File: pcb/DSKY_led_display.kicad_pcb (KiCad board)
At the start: 4 copper layers, 63.5 x 107.9 mm, 239 parts, among them J1 105133-0001, J2 3221-10-0300-00-TR, J3 TSM-104-01-L-SV, SW1 KMR241NG, U1 AP2204K-3.3, U2 LP5036, U3 LP5036, U4 LP5036, U5 LP5036, U6 ATSAMD21E18A-A, U7 LP5036, U8 LP5036, U9 TCA9543ADR

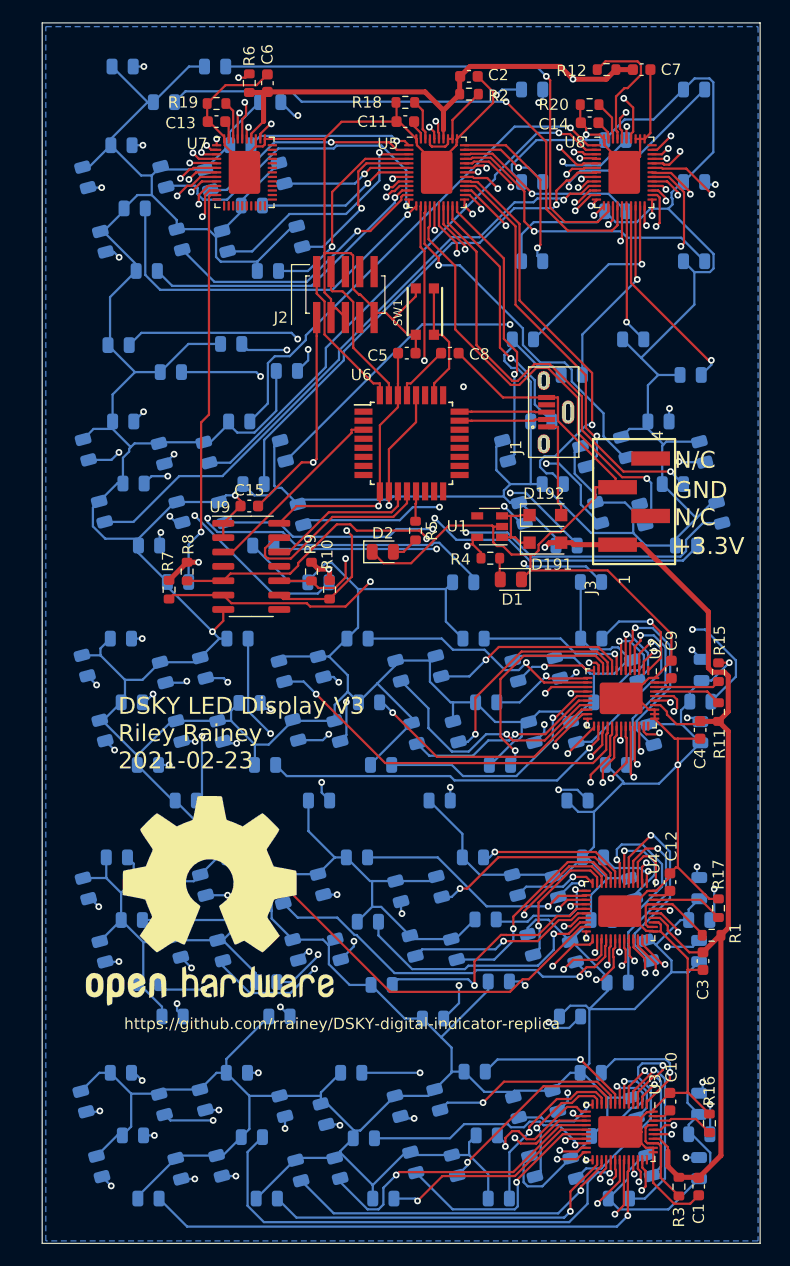
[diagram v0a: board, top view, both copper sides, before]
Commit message: V4 board
Version 4 of the PCB
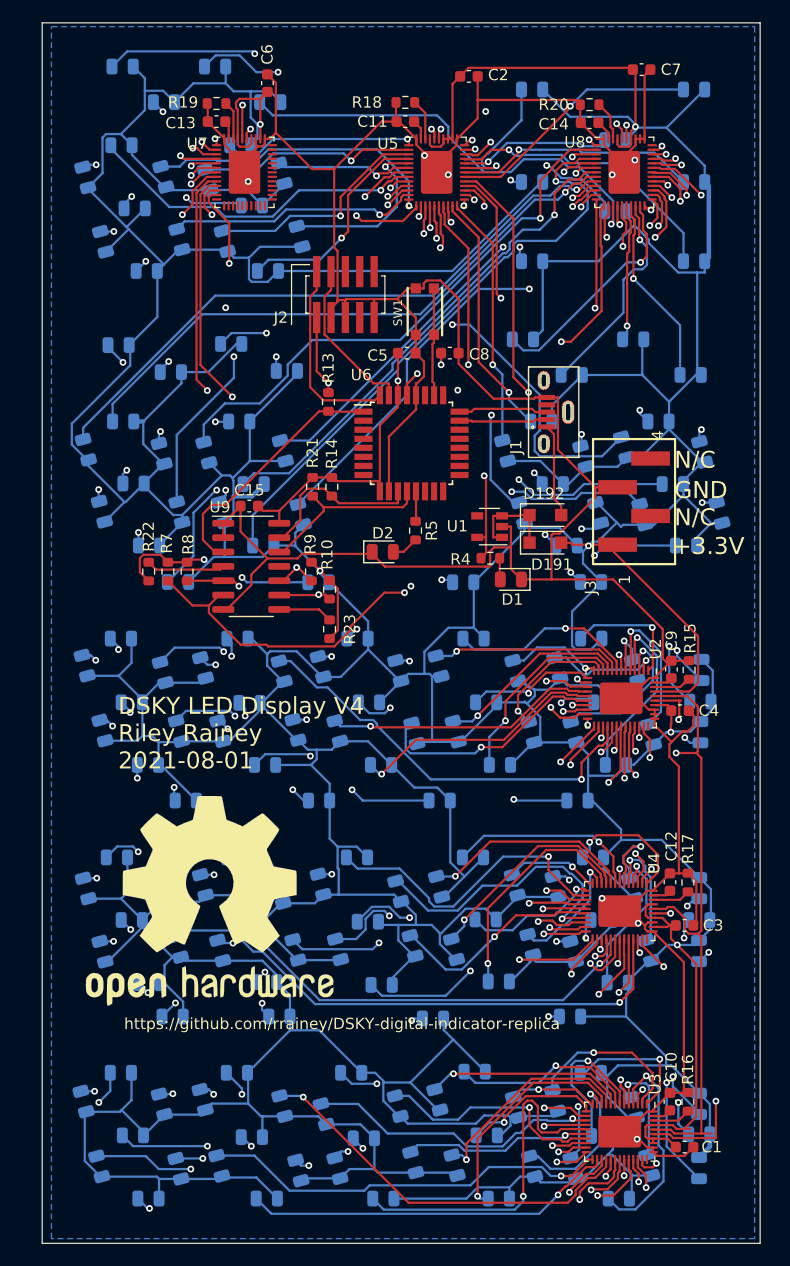
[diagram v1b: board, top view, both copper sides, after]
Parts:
- removed R1, R11, R12, R2, R3, R6: 4.7K, Resistor_SMD:R_0603_1608Metric
- added R13: 0K, Resistor_SMD:R_0603_1608Metric, F.Cu at (59.2, 66.5)
- added R14: 1K, Resistor_SMD:R_0603_1608Metric, F.Cu at (59.5, 74.0)
- added R21: 1K, Resistor_SMD:R_0603_1608Metric, F.Cu at (57.8, 74.0)
- added R22: 1K, Resistor_SMD:R_0603_1608Metric, F.Cu at (43.3, 81.5)
- added R23: 1K, Resistor_SMD:R_0603_1608Metric, F.Cu at (59.3, 86.6)
- moved C1 3.71 mm to (90.7, 132.4), turned to 0 degrees
- moved C3 3.55 mm to (90.7, 112.8), turned to 0 degrees
- moved R17 3.53 mm to (91.0, 109.0)
- moved R16 2.69 mm to (91.0, 128.4)
- moved R15 2.61 mm to (91.1, 90.2)
- moved C4 2.46 mm to (90.3, 93.8), turned to 0 degrees
- moved R7 1.60 mm to (45.0, 81.5)
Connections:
- D10 pad 1: GND -> g0bus1
- D10 pad 2: g0bus1 -> VCC
- D100 pad 1: GND -> abus32
- D100 pad 2: abus32 -> VCC
- D101 pad 1: GND -> abus3
- D101 pad 2: abus3 -> VCC
- D102 pad 1: GND -> sabus2
- D102 pad 2: sabus2 -> VCC
- D103 pad 1: GND -> abus10
- D103 pad 2: abus10 -> VCC
- D104 pad 1: GND -> abus17
- D104 pad 2: abus17 -> VCC
- D105 pad 1: GND -> abus24
- D105 pad 2: abus24 -> VCC
- D106 pad 1: GND -> abus31
- D106 pad 2: abus31 -> VCC
- D107 pad 1: GND -> g5bus0
- D107 pad 2: g5bus0 -> VCC
- D108 pad 1: GND -> g5bus1
- D108 pad 2: g5bus1 -> VCC
- D109 pad 1: GND -> g5bus2
- D109 pad 2: g5bus2 -> VCC
- D11 pad 1: GND -> g0bus6
- D11 pad 2: g0bus6 -> VCC
- D110 pad 1: GND -> g5bus3
- D110 pad 2: g5bus3 -> VCC
- D111 pad 1: GND -> bbus0
- D111 pad 2: bbus0 -> VCC
- D112 pad 1: GND -> sbbus0
- D112 pad 2: sbbus0 -> VCC
- D113 pad 1: GND -> bbus7
- D113 pad 2: bbus7 -> VCC
- D114 pad 1: GND -> bbus14
- D114 pad 2: bbus14 -> VCC
- D115 pad 1: GND -> bbus21
- D115 pad 2: bbus21 -> VCC
- D116 pad 1: GND -> bbus28
- D116 pad 2: bbus28 -> VCC
- D117 pad 1: GND -> bbus5
- D117 pad 2: bbus5 -> VCC
- D118 pad 1: GND -> bbus1
- D118 pad 2: bbus1 -> VCC
- D119 pad 1: GND -> bbus12
- D119 pad 2: bbus12 -> VCC
- D12 pad 1: GND -> g0bus5
- D12 pad 2: g0bus5 -> VCC
- D120 pad 1: GND -> bbus19
- D120 pad 2: bbus19 -> VCC
- D121 pad 1: GND -> bbus8
- D121 pad 2: bbus8 -> VCC
- D122 pad 1: GND -> bbus15
- D122 pad 2: bbus15 -> VCC
- D123 pad 1: GND -> bbus26
- D123 pad 2: bbus26 -> VCC
- D124 pad 1: GND -> bbus33
- D124 pad 2: bbus33 -> VCC
- D125 pad 1: GND -> bbus22
- D125 pad 2: bbus22 -> VCC
- D126 pad 1: GND -> bbus29
- D126 pad 2: bbus29 -> VCC
- D127 pad 1: GND -> sbbus1
- D127 pad 2: sbbus1 -> VCC
- D128 pad 1: GND -> bbus6
- D128 pad 2: bbus6 -> VCC
- D129 pad 1: GND -> bbus13
- D129 pad 2: bbus13 -> VCC
- D13 pad 1: GND -> g0bus4
- D13 pad 2: g0bus4 -> VCC
- D130 pad 1: GND -> bbus20
- D130 pad 2: bbus20 -> VCC
- D131 pad 1: GND -> bbus27
- D131 pad 2: bbus27 -> VCC
- D132 pad 1: GND -> bbus34
- D132 pad 2: bbus34 -> VCC
- D133 pad 1: GND -> bbus2
- D133 pad 2: bbus2 -> VCC
- D134 pad 1: GND -> bbus4
- D134 pad 2: bbus4 -> VCC
- D135 pad 1: GND -> bbus9
- D135 pad 2: bbus9 -> VCC
- D136 pad 1: GND -> bbus16
- D136 pad 2: bbus16 -> VCC
- D137 pad 1: GND -> bbus11
- D137 pad 2: bbus11 -> VCC
- D138 pad 1: GND -> bbus18
- D138 pad 2: bbus18 -> VCC
- D139 pad 1: GND -> bbus23
- D139 pad 2: bbus23 -> VCC
- D14 pad 1: GND -> g0bus7
- D14 pad 2: g0bus7 -> VCC
- D140 pad 1: GND -> bbus30
- D140 pad 2: bbus30 -> VCC
- D141 pad 1: GND -> bbus25
- D141 pad 2: bbus25 -> VCC
- D142 pad 1: GND -> bbus32
- D142 pad 2: bbus32 -> VCC
- D143 pad 1: GND -> sbbus2
- D143 pad 2: sbbus2 -> VCC
- D144 pad 1: GND -> bbus3
- D144 pad 2: bbus3 -> VCC
- D145 pad 1: GND -> bbus10
- D145 pad 2: bbus10 -> VCC
- D146 pad 1: GND -> bbus17
- D146 pad 2: bbus17 -> VCC
- D147 pad 1: GND -> bbus24
- D147 pad 2: bbus24 -> VCC
- D148 pad 1: GND -> bbus31
- D148 pad 2: bbus31 -> VCC
- D149 pad 1: GND -> g6bus0
- D149 pad 2: g6bus0 -> VCC
- D15 pad 1: GND -> dbus0
- D15 pad 2: dbus0 -> VCC
- D150 pad 1: GND -> g6bus1
- D150 pad 2: g6bus1 -> VCC
- D151 pad 1: GND -> g6bus2
- D151 pad 2: g6bus2 -> VCC
- D152 pad 1: GND -> g6bus3
- D152 pad 2: g6bus3 -> VCC
- D153 pad 1: GND -> scbus0
- D153 pad 2: scbus0 -> VCC
- D154 pad 1: GND -> cbus0
- D154 pad 2: cbus0 -> VCC
- D155 pad 1: GND -> cbus7
- D155 pad 2: cbus7 -> VCC
- D156 pad 1: GND -> cbus14
- D156 pad 2: cbus14 -> VCC
- D157 pad 1: GND -> cbus21
- D157 pad 2: cbus21 -> VCC
- D158 pad 1: GND -> cbus28
- D158 pad 2: cbus28 -> VCC
- D159 pad 1: GND -> cbus5
- D159 pad 2: cbus5 -> VCC
- D16 pad 1: GND -> dbus7
- D16 pad 2: dbus7 -> VCC
- D160 pad 1: GND -> cbus1
- D160 pad 2: cbus1 -> VCC
- D161 pad 1: GND -> cbus12
- D161 pad 2: cbus12 -> VCC
- D162 pad 1: GND -> cbus19
- D162 pad 2: cbus19 -> VCC
- D163 pad 1: GND -> scbus1
- D163 pad 2: scbus1 -> VCC
- D164 pad 1: GND -> cbus8
- D164 pad 2: cbus8 -> VCC
- D165 pad 1: GND -> cbus15
- D165 pad 2: cbus15 -> VCC
- D166 pad 1: GND -> cbus26
- D166 pad 2: cbus26 -> VCC
- D167 pad 1: GND -> cbus33
- D167 pad 2: cbus33 -> VCC
- D168 pad 1: GND -> cbus22
- D168 pad 2: cbus22 -> VCC
- D169 pad 1: GND -> cbus29
- D169 pad 2: cbus29 -> VCC
- D17 pad 1: GND -> dbus5
- D17 pad 2: dbus5 -> VCC
- D170 pad 1: GND -> cbus6
- D170 pad 2: cbus6 -> VCC
- D171 pad 1: GND -> cbus13
- D171 pad 2: cbus13 -> VCC
- D172 pad 1: GND -> cbus20
- D172 pad 2: cbus20 -> VCC
- D173 pad 1: GND -> cbus27
- D173 pad 2: cbus27 -> VCC
- D174 pad 1: GND -> cbus34
- D174 pad 2: cbus34 -> VCC
- D175 pad 1: GND -> cbus2
- D175 pad 2: cbus2 -> VCC
- D176 pad 1: GND -> scbus2
- D176 pad 2: scbus2 -> VCC
- D177 pad 1: GND -> cbus4
- D177 pad 2: cbus4 -> VCC
- D178 pad 1: GND -> cbus9
- D178 pad 2: cbus9 -> VCC
- D179 pad 1: GND -> cbus16
- D179 pad 2: cbus16 -> VCC
- D18 pad 1: GND -> dbus12
- D18 pad 2: dbus12 -> VCC
- D180 pad 1: GND -> cbus11
- D180 pad 2: cbus11 -> VCC
- D181 pad 1: GND -> cbus18
- D181 pad 2: cbus18 -> VCC
- D182 pad 1: GND -> cbus23
- D182 pad 2: cbus23 -> VCC
- D183 pad 1: GND -> cbus30
- D183 pad 2: cbus30 -> VCC
- D184 pad 1: GND -> cbus25
- D184 pad 2: cbus25 -> VCC
- D185 pad 1: GND -> cbus32
- D185 pad 2: cbus32 -> VCC
- D186 pad 1: GND -> cbus3
- D186 pad 2: cbus3 -> VCC
- D187 pad 1: GND -> cbus10
- D187 pad 2: cbus10 -> VCC
- D188 pad 1: GND -> cbus17
- D188 pad 2: cbus17 -> VCC
- D189 pad 1: GND -> cbus24
- D189 pad 2: cbus24 -> VCC
- D19 pad 1: GND -> dbus1
- D19 pad 2: dbus1 -> VCC
- D190 pad 1: GND -> cbus31
- D190 pad 2: cbus31 -> VCC
- D20 pad 1: GND -> dbus8
- D20 pad 2: dbus8 -> VCC
- D21 pad 1: GND -> dbus6
- D21 pad 2: dbus6 -> VCC
- D22 pad 1: GND -> dbus13
- D22 pad 2: dbus13 -> VCC
- D23 pad 1: GND -> dbus2
- D23 pad 2: dbus2 -> VCC
- D24 pad 1: GND -> dbus9
- D24 pad 2: dbus9 -> VCC
- D25 pad 1: GND -> dbus4
- D25 pad 2: dbus4 -> VCC
- D26 pad 1: GND -> dbus11
- D26 pad 2: dbus11 -> VCC
- D27 pad 1: GND -> dbus3
- D27 pad 2: dbus3 -> VCC
- D28 pad 1: GND -> dbus10
- D28 pad 2: dbus10 -> VCC
- D29 pad 1: GND -> g2bus0
- D29 pad 2: g2bus0 -> VCC
- D3 pad 1: GND -> g0bus0
- D3 pad 2: g0bus0 -> VCC
- D30 pad 1: GND -> g2bus3
- D30 pad 2: g2bus3 -> VCC
- D31 pad 1: GND -> g3bus0
- D31 pad 2: g3bus0 -> VCC
- D32 pad 1: GND -> g3bus3
- D32 pad 2: g3bus3 -> VCC
- D33 pad 1: GND -> g2bus1
- D33 pad 2: g2bus1 -> VCC
- D34 pad 1: GND -> g2bus2
- D34 pad 2: g2bus2 -> VCC
- D35 pad 1: GND -> g3bus1
- D35 pad 2: g3bus1 -> VCC
- D36 pad 1: GND -> g3bus2
- D36 pad 2: g3bus2 -> VCC
- D37 pad 1: GND -> ebus0
- D37 pad 2: ebus0 -> VCC
- D38 pad 1: GND -> ebus7
- D38 pad 2: ebus7 -> VCC
- D39 pad 1: GND -> fbus0
- D39 pad 2: fbus0 -> VCC
- D4 pad 1: GND -> g0bus2
- D4 pad 2: g0bus2 -> VCC
- D40 pad 1: GND -> fbus7
- D40 pad 2: fbus7 -> VCC
- D41 pad 1: GND -> ebus5
- D41 pad 2: ebus5 -> VCC
- D42 pad 1: GND -> ebus12
- D42 pad 2: ebus12 -> VCC
- D43 pad 1: GND -> ebus1
- D43 pad 2: ebus1 -> VCC
- D44 pad 1: GND -> ebus8
- D44 pad 2: ebus8 -> VCC
- D45 pad 1: GND -> fbus5
- D45 pad 2: fbus5 -> VCC
- D46 pad 1: GND -> fbus12
- D46 pad 2: fbus12 -> VCC
- D47 pad 1: GND -> fbus1
- D47 pad 2: fbus1 -> VCC
- D48 pad 1: GND -> fbus8
- D48 pad 2: fbus8 -> VCC
- D49 pad 1: GND -> ebus6
- D49 pad 2: ebus6 -> VCC
- D5 pad 1: GND -> g1bus0
- D5 pad 2: g1bus0 -> VCC
- D50 pad 1: GND -> ebus13
- D50 pad 2: ebus13 -> VCC
- D51 pad 1: GND -> fbus6
- D51 pad 2: fbus6 -> VCC
- D52 pad 1: GND -> fbus13
- D52 pad 2: fbus13 -> VCC
- D53 pad 1: GND -> ebus2
- D53 pad 2: ebus2 -> VCC
- D54 pad 1: GND -> ebus9
- D54 pad 2: ebus9 -> VCC
- D55 pad 1: GND -> ebus4
- D55 pad 2: ebus4 -> VCC
- D56 pad 1: GND -> VCC
- D57 pad 1: GND -> fbus2
- D57 pad 2: fbus2 -> VCC
- D58 pad 1: GND -> fbus9
- D58 pad 2: fbus9 -> VCC
- D59 pad 1: GND -> fbus4
- D59 pad 2: fbus4 -> VCC
- D6 pad 1: GND -> g1bus3
- D6 pad 2: g1bus3 -> VCC
- D60 pad 1: GND -> fbus11
- D60 pad 2: fbus11 -> VCC
- D61 pad 1: GND -> ebus3
- D61 pad 2: ebus3 -> VCC
- D62 pad 1: GND -> ebus10
- D62 pad 2: ebus10 -> VCC
- D63 pad 1: GND -> fbus3
- D63 pad 2: fbus3 -> VCC
- D64 pad 1: GND -> fbus10
- D64 pad 2: fbus10 -> VCC
- D65 pad 1: GND -> g4bus0
- D65 pad 2: g4bus0 -> VCC
- D66 pad 1: GND -> g4bus1
- D66 pad 2: g4bus1 -> VCC
- D67 pad 1: GND -> g4bus2
- D67 pad 2: g4bus2 -> VCC
- D68 pad 1: GND -> g4bus3
- D68 pad 2: g4bus3 -> VCC
- D69 pad 1: GND -> abus0
- D69 pad 2: abus0 -> VCC
- D7 pad 1: GND -> g0bus3
- D7 pad 2: g0bus3 -> VCC
- D70 pad 1: GND -> abus7
- D70 pad 2: abus7 -> VCC
- D71 pad 1: GND -> abus14
- D71 pad 2: abus14 -> VCC
- D72 pad 1: GND -> abus21
- D72 pad 2: abus21 -> VCC
- D73 pad 1: GND -> abus28
- D73 pad 2: abus28 -> VCC
- D74 pad 1: GND -> sabus0
- D74 pad 2: sabus0 -> VCC
- D75 pad 1: GND -> abus5
- D75 pad 2: abus5 -> VCC
- D76 pad 1: GND -> abus1
- D76 pad 2: abus1 -> VCC
- D77 pad 1: GND -> abus12
- D77 pad 2: abus12 -> VCC
- D78 pad 1: GND -> abus19
- D78 pad 2: abus19 -> VCC
- D79 pad 1: GND -> abus8
- D79 pad 2: abus8 -> VCC
- D8 pad 1: GND -> g1bus1
- D8 pad 2: g1bus1 -> VCC
- D80 pad 1: GND -> abus15
- D80 pad 2: abus15 -> VCC
- D81 pad 1: GND -> abus26
- D81 pad 2: abus26 -> VCC
- D82 pad 1: GND -> abus33
- D82 pad 2: abus33 -> VCC
- D83 pad 1: GND -> abus22
- D83 pad 2: abus22 -> VCC
- D84 pad 1: GND -> abus29
- D84 pad 2: abus29 -> VCC
- D85 pad 1: GND -> abus6
- D85 pad 2: abus6 -> VCC
- D86 pad 1: GND -> sabus1
- D86 pad 2: sabus1 -> VCC
- D87 pad 1: GND -> abus13
- D87 pad 2: abus13 -> VCC
- D88 pad 1: GND -> abus20
- D88 pad 2: abus20 -> VCC
- D89 pad 1: GND -> abus27
- D89 pad 2: abus27 -> VCC
- D9 pad 1: GND -> g1bus2
- D9 pad 2: g1bus2 -> VCC
- D90 pad 1: GND -> abus34
- D90 pad 2: abus34 -> VCC
- D91 pad 1: GND -> abus2
- D91 pad 2: abus2 -> VCC
- D92 pad 1: GND -> abus4
- D92 pad 2: abus4 -> VCC
- D93 pad 1: GND -> abus9
- D93 pad 2: abus9 -> VCC
- D94 pad 1: GND -> abus16
- D94 pad 2: abus16 -> VCC
- D95 pad 1: GND -> abus11
- D95 pad 2: abus11 -> VCC
- D96 pad 1: GND -> abus18
- D96 pad 2: abus18 -> VCC
- D97 pad 1: GND -> abus23
- D97 pad 2: abus23 -> VCC
- D98 pad 1: GND -> abus30
- D98 pad 2: abus30 -> VCC
- D99 pad 1: GND -> abus25
- D99 pad 2: abus25 -> VCC
- J1 pad 4: Net-(J1-Pad4) -> (no net)
- J1 pad S2: Net-(J1-PadS2) -> (no net)
- J2 pad 10: Net-(J2-Pad10) -> (no net)
- J2 pad 6: Net-(J2-Pad6) -> (no net)
- J2 pad 7: Net-(J2-Pad7) -> (no net)
- J2 pad 8: Net-(J2-Pad8) -> (no net)
- J3 pad 2: Net-(J3-Pad2) -> (no net)
- J3 pad 4: Net-(J3-Pad4) -> (no net)
- U1 pad 4: Net-(U1-Pad4) -> (no net)
- U2 pad 36: Net-(U2-Pad36) -> (no net)
- U2 pad 43: Net-(R11-Pad2) -> VCC
- U3 pad 36: Net-(U3-Pad36) -> (no net)
- U3 pad 39: Net-(R3-Pad2) -> VCC
- U3 pad 43: Net-(R3-Pad2) -> VCC
- U4 pad 36: Net-(U4-Pad36) -> (no net)
- U4 pad 38: Net-(R1-Pad2) -> VCC
- U4 pad 43: Net-(R1-Pad2) -> VCC
- U5 pad 38: Net-(R2-Pad2) -> VCC
- U5 pad 39: Net-(R2-Pad2) -> VCC
- U5 pad 43: Net-(R2-Pad2) -> VCC
- U6 pad 1: Net-(U6-Pad1) -> /BRESET
- U6 pad 14: Net-(U6-Pad14) -> (no net)
- U6 pad 15: Net-(U6-Pad15) -> (no net)
- U6 pad 16: Net-(U6-Pad16) -> (no net)
- U6 pad 17: Net-(U6-Pad17) -> (no net)
- U6 pad 18: Net-(U6-Pad18) -> (no net)
- U6 pad 19: Net-(U6-Pad19) -> (no net)
- U6 pad 2: Net-(U6-Pad2) -> (no net)
- U6 pad 20: Net-(U6-Pad20) -> (no net)
- U6 pad 21: Net-(U6-Pad21) -> (no net)
- U6 pad 22: Net-(U6-Pad22) -> (no net)
- U6 pad 25: Net-(U6-Pad25) -> (no net)
- U6 pad 27: Net-(U6-Pad27) -> (no net)
- U6 pad 3: /BRESET -> (no net)
- U6 pad 4: Net-(U6-Pad4) -> (no net)
- U6 pad 5: Net-(U6-Pad5) -> (no net)
- U6 pad 6: Net-(U6-Pad6) -> (no net)
- U6 pad 7: Net-(U6-Pad7) -> (no net)
- U6 pad 8: Net-(U6-Pad8) -> (no net)
- U7 pad 13: Net-(U7-Pad13) -> (no net)
- U7 pad 14: Net-(U7-Pad14) -> (no net)
- U7 pad 15: Net-(U7-Pad15) -> (no net)
- U7 pad 16: Net-(U7-Pad16) -> (no net)
- U7 pad 17: Net-(U7-Pad17) -> (no net)
- U7 pad 18: Net-(U7-Pad18) -> (no net)
- U7 pad 19: Net-(U7-Pad19) -> (no net)
- U7 pad 20: Net-(U7-Pad20) -> (no net)
- U7 pad 21: Net-(U7-Pad21) -> (no net)
- U7 pad 22: Net-(U7-Pad22) -> (no net)
- U7 pad 23: Net-(U7-Pad23) -> (no net)
- U7 pad 24: Net-(U7-Pad24) -> (no net)
- U7 pad 25: Net-(U7-Pad25) -> (no net)
- U7 pad 26: Net-(U7-Pad26) -> (no net)
- U7 pad 27: Net-(U7-Pad27) -> (no net)
- U7 pad 28: Net-(U7-Pad28) -> (no net)
- U7 pad 29: Net-(U7-Pad29) -> (no net)
- U7 pad 30: Net-(U7-Pad30) -> (no net)
- U7 pad 31: Net-(U7-Pad31) -> (no net)
- U7 pad 32: Net-(U7-Pad32) -> (no net)
- U7 pad 33: Net-(U7-Pad33) -> (no net)
- U7 pad 34: Net-(U7-Pad34) -> (no net)
- U7 pad 35: Net-(U7-Pad35) -> (no net)
- U7 pad 36: Net-(U7-Pad36) -> (no net)
- U7 pad 38: Net-(R6-Pad2) -> VCC
- U7 pad 43: Net-(R6-Pad2) -> VCC
- U8 pad 36: Net-(U8-Pad36) -> (no net)
- U8 pad 43: Net-(R12-Pad2) -> VCC
- U9 pad 11: Net-(U9-Pad11) -> (no net)
- U9 pad 12: /3SDA -> /3SCL
- U9 pad 13: /3SCL -> /3SDA
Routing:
- net GND: track 1226.0 -> 300.1 mm, vias 7 -> 8
- net VCC: track 226.6 -> 1083.5 mm, vias 5 -> 7
- net fbus0: track 44.5 -> 64.6 mm, vias 1 -> 2
- net g4bus0: track 79.5 -> 60.1 mm
- net /SCL0: track 138.4 -> 155.7 mm, vias 5 -> 3
- net abus28: track 65.0 -> 51.0 mm
- net Net-(R12-Pad2): track 12.0 -> 0.00 mm
- net Net-(R6-Pad2): track 11.6 -> 0.00 mm, vias 3 -> 0
- net dbus6: track 14.2 -> 25.7 mm, vias 1 -> 2
- net cbus17: track 19.7 -> 30.8 mm
- net ebus4: track 55.2 -> 44.3 mm, vias 2 -> 3
- net g4bus1: track 57.5 -> 47.1 mm
- net fbus10: track 56.8 -> 66.1 mm
- net fbus4: track 54.7 -> 45.4 mm
- net /SCL1: track 93.7 -> 85.1 mm
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- added copper zone on In1.Cu, net GND
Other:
- board text added: "DSKY LED Display V4 Riley Rainey 2021-08-01"
- board text removed: "DSKY LED Display V3 Riley Rainey 2021-02-23"
